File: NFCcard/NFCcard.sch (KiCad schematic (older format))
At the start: 2 parts

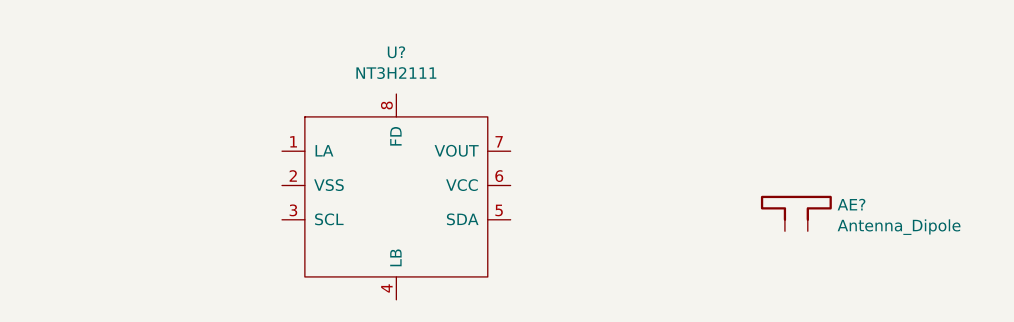
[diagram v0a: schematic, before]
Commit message: Finnally Imported
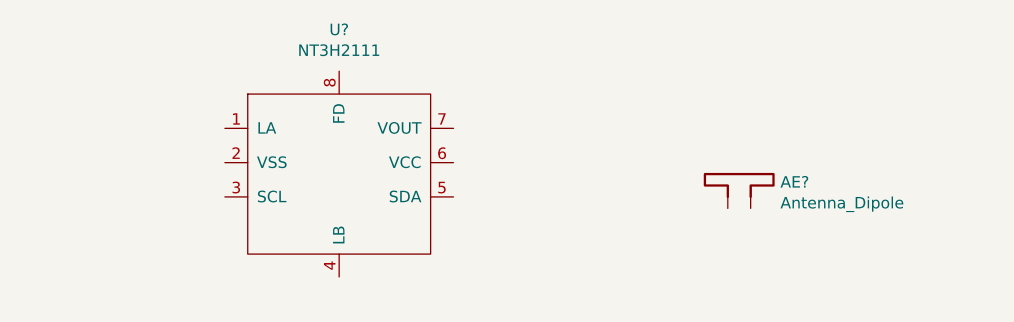
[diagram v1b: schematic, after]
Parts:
- AE?: footprint (none) -> NFCcard:NFCantenna
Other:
- moved on the sheet: AE?, U?
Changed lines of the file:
@@
 L Me-NFC:NT3H2111 U?
 U 1 1 5F8857C9
-P 3850 3150
-F 0 "U?" H 3850 4231 50  0000 C CNN
-F 1 "NT3H2111" H 3850 4140 50  0000 C CNN
-F 2 "Package_SO:TSSOP-8_3x3mm_P0.65mm" H 4700 3000 50  0001 C CNN
-F 3 "" H 3850 3150 50  0001 C CNN
-	1    3850 3150
+P 3600 3050
+F 0 "U?" H 3600 4131 50  0000 C CNN
+F 1 "NT3H2111" H 3600 4040 50  0000 C CNN
+F 2 "Package_SO:TSSOP-8_3x3mm_P0.65mm" H 4450 2900 50  0001 C CNN
+F 3 "" H 3600 3050 50  0001 C CNN
+	1    3600 3050
 	1    0    0    -1
 $EndComp
@@
 L Device:Antenna_Dipole AE?
 U 1 1 5F88B0DD
-P 5550 2650
-F 0 "AE?" H 5780 2564 50  0000 L CNN
-F 1 "Antenna_Dipole" H 5780 2473 50  0000 L CNN
-F 2 "" H 5550 2650 50  0001 C CNN
-F 3 "~" H 5550 2650 50  0001 C CNN
-	1    5550 2650
+P 5300 2550
+F 0 "AE?" H 5530 2464 50  0000 L CNN
+F 1 "Antenna_Dipole" H 5530 2373 50  0000 L CNN
+F 2 "NFCcard:NFCantenna" H 5300 2550 50  0001 C CNN
+F 3 "~" H 5300 2550 50  0001 C CNN
+	1    5300 2550
 	1    0    0    -1
 $EndComp

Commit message: Layout
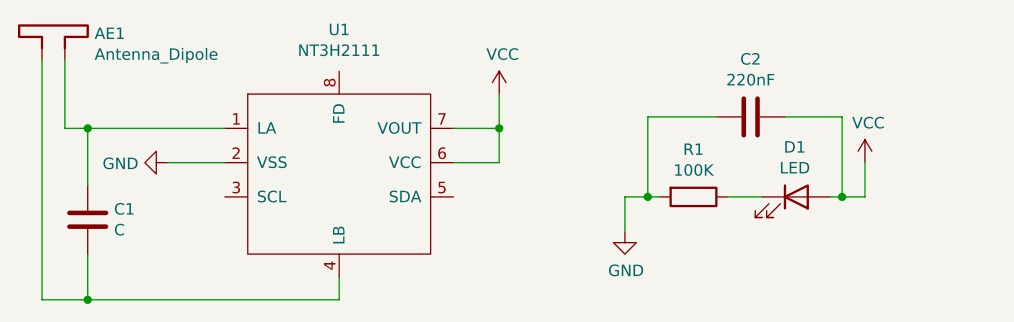
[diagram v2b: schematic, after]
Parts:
- added C1: C, Capacitor_SMD:C_0603_1608Metric, symbol Device:C
- added C2: 220nF, Capacitor_SMD:C_0603_1608Metric, symbol Device:C
- added D1: LED, LED_SMD:LED_0603_1608Metric, symbol Device:LED
- added R1: 100K, Capacitor_SMD:C_0603_1608Metric, symbol Device:R
- gave numbers to parts that had none: 2
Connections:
- net at U1.1 (LA): now also AE1.2, C1.2
- net GND: now reaches U1.2 (VSS)
- net GND: now also C2.2, R1.2
- net at U1.4 (LB): now also AE1.1, C1.1
- net VCC: now reaches U1.6 (VCC)
- net VCC: now also U1.7 (VOUT), C2.1, D1.2 (A)
- new net: D1.1 (K), R1.1
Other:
- moved on the sheet: AE1
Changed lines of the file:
@@
 $EndDescr
 $Comp
-L Me-NFC:NT3H2111 U?
+L Me-NFC:NT3H2111 U1
 U 1 1 5F8857C9
 P 3600 3050
-F 0 "U?" H 3600 4131 50  0000 C CNN
+F 0 "U1" H 3600 4131 50  0000 C CNN
 F 1 "NT3H2111" H 3600 4040 50  0000 C CNN
 F 2 "Package_SO:TSSOP-8_3x3mm_P0.65mm" H 4450 2900 50  0001 C CNN
@@
 $EndComp
 $Comp
-L Device:Antenna_Dipole AE?
+L Device:Antenna_Dipole AE1
 U 1 1 5F88B0DD
-P 5300 2550
-F 0 "AE?" H 5530 2464 50  0000 L CNN
-F 1 "Antenna_Dipole" H 5530 2373 50  0000 L CNN
-F 2 "NFCcard:NFCantenna" H 5300 2550 50  0001 C CNN
-F 3 "~" H 5300 2550 50  0001 C CNN
-	1    5300 2550
+P 2300 1900
+F 0 "AE1" H 2530 1814 50  0000 L CNN
+F 1 "Antenna_Dipole" H 2530 1723 50  0000 L CNN
+F 2 "NFCcard:NFCantenna" H 2300 1900 50  0001 C CNN
+F 3 "~" H 2300 1900 50  0001 C CNN
+	1    2300 1900
 	1    0    0    -1
 $EndComp
+$Comp
+L Device:C C2
+U 1 1 5F88FD22
+P 5400 2350
+F 0 "C2" V 5148 2350 50  0000 C CNN
+F 1 "220nF" V 5239 2350 50  0000 C CNN
+F 2 "Capacitor_SMD:C_0603_1608Metric" H 5438 2200 50  0001 C CNN
+F 3 "~" H 5400 2350 50  0001 C CNN
+	1    5400 2350
+	0    1    1    0
+$EndComp
+$Comp
+L Device:R R1
+U 1 1 5F8918EF
+P 5150 2700
+F 0 "R1" V 4943 2700 50  0000 C CNN
+F 1 "100K" V 5034 2700 50  0000 C CNN
+F 2 "Capacitor_SMD:C_0603_1608Metric" V 5080 2700 50  0001 C CNN
+F 3 "~" H 5150 2700 50  0001 C CNN
+	1    5150 2700
+	0    1    1    0
+$EndComp
+$Comp
+L Device:LED D1
+U 1 1 5F893394
+P 5600 2700
+F 0 "D1" H 5593 2917 50  0000 C CNN
+F 1 "LED" H 5593 2826 50  0000 C CNN
+F 2 "LED_SMD:LED_0603_1608Metric" H 5600 2700 50  0001 C CNN
+F 3 "~" H 5600 2700 50  0001 C CNN
+	1    5600 2700
+	1    0    0    -1
+$EndComp
+Wire Wire Line
+	2300 2100 2300 3150
+Wire Wire Line
+	2300 3150 2500 3150
+Wire Wire Line
+	3600 3150 3600 3050
+Wire Wire Line
+	3100 2400 2500 2400
+Wire Wire Line
+	2400 2400 2400 2100
+$Comp
+L power:GND #PWR0101
+U 1 1 5F8987A2
+P 2850 2550
+F 0 "#PWR0101" H 2850 2300 50  0001 C CNN
+F 1 "GND" V 2855 2422 50  0000 R CNN
+F 2 "" H 2850 2550 50  0001 C CNN
+F 3 "" H 2850 2550 50  0001 C CNN
+	1    2850 2550
+	0    1    1    0
+$EndComp
+Wire Wire Line
+	2850 2550 3100 2550
+$Comp
+L power:VCC #PWR0102
+U 1 1 5F89A687
+P 4300 2250
+F 0 "#PWR0102" H 4300 2100 50  0001 C CNN
+F 1 "VCC" H 4315 2423 50  0000 C CNN
+F 2 "" H 4300 2250 50  0001 C CNN
+F 3 "" H 4300 2250 50  0001 C CNN
+	1    4300 2250
+	1    0    0    -1
+$EndComp
+Wire Wire Line
+	4300 2250 4300 2400
+Wire Wire Line
+	4300 2400 4100 2400
+Wire Wire Line
+	4300 2400 4300 2550
+Wire Wire Line
+	4300 2550 4100 2550
+Connection ~ 4300 2400
+$Comp
+L Device:C C1
+U 1 1 5F89C228
+P 2500 2800
+F 0 "C1" H 2385 2754 50  0000 R CNN
+F 1 "C" H 2385 2845 50  0000 R CNN
+F 2 "Capacitor_SMD:C_0603_1608Metric" H 2538 2650 50  0001 C CNN
+F 3 "~" H 2500 2800 50  0001 C CNN
+	1    2500 2800
+	-1   0    0    1
+$EndComp
+Wire Wire Line
+	2500 2650 2500 2400
+Connection ~ 2500 2400
+Wire Wire Line
+	2500 2400 2400 2400
+Wire Wire Line
+	2500 2950 2500 3150
+Connection ~ 2500 3150
+Wire Wire Line
+	2500 3150 3600 3150
+$Comp
+L power:GND #PWR0103
+U 1 1 5F8A1582
+P 4850 2850
+F 0 "#PWR0103" H 4850 2600 50  0001 C CNN
+F 1 "GND" H 4855 2677 50  0000 C CNN
+F 2 "" H 4850 2850 50  0001 C CNN
+F 3 "" H 4850 2850 50  0001 C CNN
+	1    4850 2850
+	1    0    0    -1
+$EndComp
+$Comp
+L power:VCC #PWR0104
+U 1 1 5F8A2529
+P 5900 2550
+F 0 "#PWR0104" H 5900 2400 50  0001 C CNN
+F 1 "VCC" H 5915 2723 50  0000 C CNN
+F 2 "" H 5900 2550 50  0001 C CNN
+F 3 "" H 5900 2550 50  0001 C CNN
+	1    5900 2550
+	1    0    0    -1
+$EndComp
+Wire Wire Line
+	5900 2550 5900 2700
+Wire Wire Line
+	5900 2700 5800 2700
+Wire Wire Line
+	5450 2700 5300 2700
+Wire Wire Line
+	5000 2700 4950 2700
+Wire Wire Line
+	4850 2700 4850 2850
+Wire Wire Line
+	5250 2350 4950 2350
+Wire Wire Line
+	4950 2350 4950 2700
+Connection ~ 4950 2700
+Wire Wire Line
+	4950 2700 4850 2700
+Wire Wire Line
+	5550 2350 5800 2350
+Wire Wire Line
+	5800 2350 5800 2700
+Connection ~ 5800 2700
+Wire Wire Line
+	5800 2700 5750 2700
 $EndSCHEMATC
